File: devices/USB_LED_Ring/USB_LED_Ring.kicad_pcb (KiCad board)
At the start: 2 copper layers, 94.5 x 75 mm, 91 parts, among them J1 JST SH 3 Vert, J2 USB_B_Micro, J3 JST SH 3 Vert, J4 .100, U1 TPS923610, U2 TLV75733PDBV, U3 RP2354A, U4 TPS25947xx, Y1 ABM8-272-T3

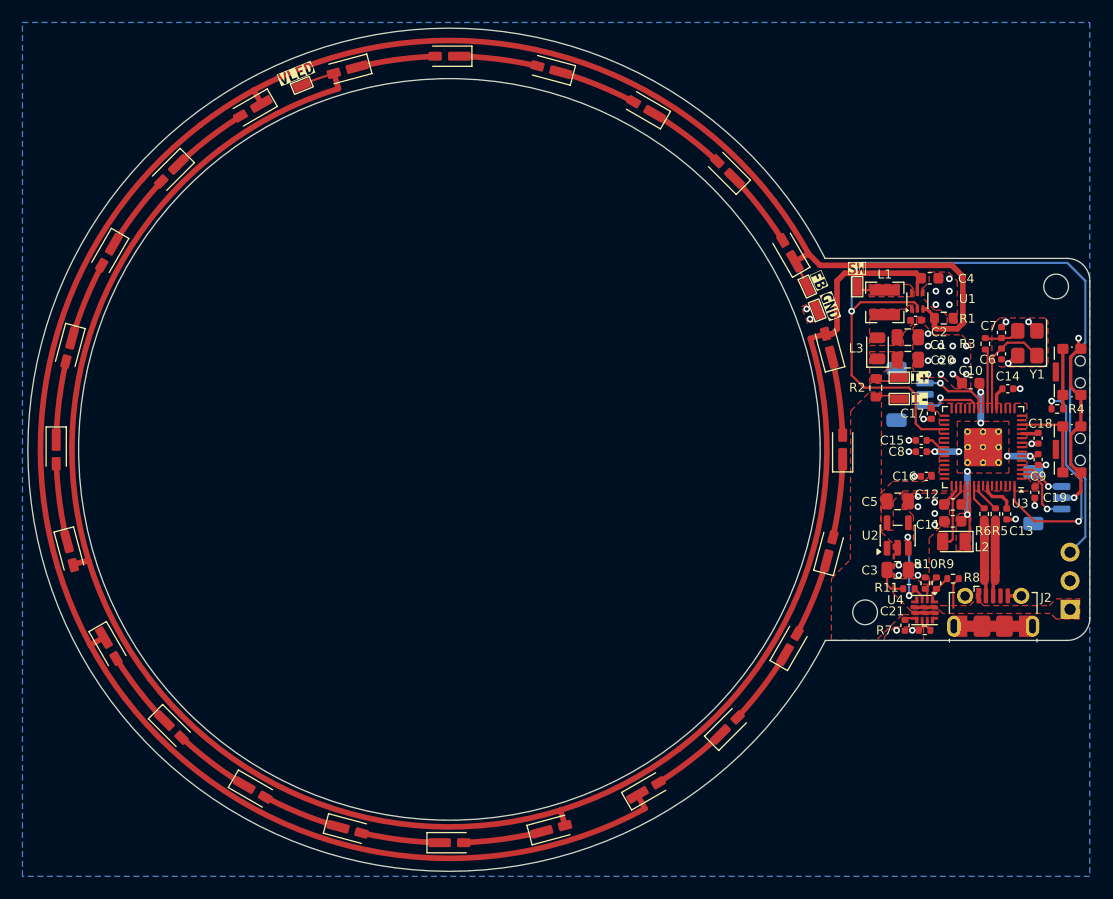
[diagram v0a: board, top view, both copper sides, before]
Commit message: Finsihes version A.0 of the BLE sensor
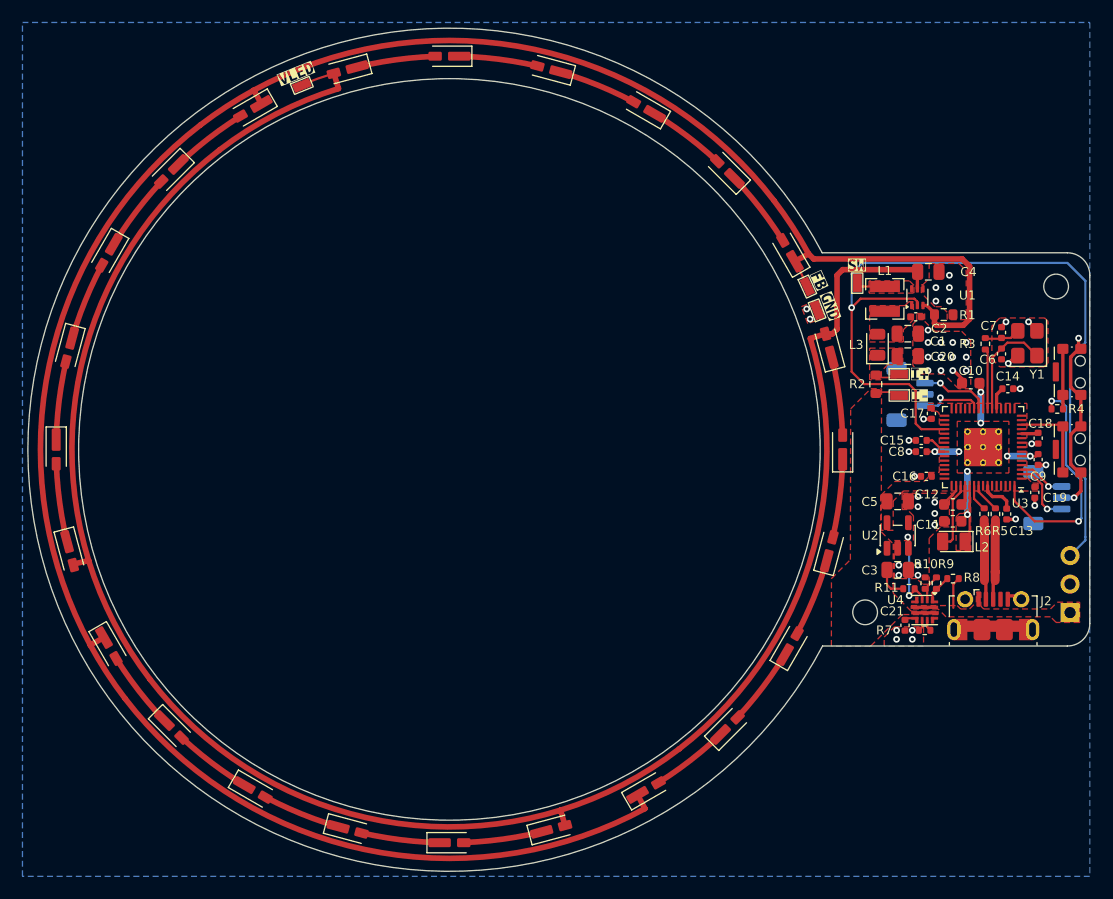
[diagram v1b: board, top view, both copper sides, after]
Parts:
- C4: value 1u -> 2u2; footprint Capacitor_SMD:C_0603_1608Metric -> Capacitor_SMD:C_0805_2012Metric
- moved C4 0.59 mm to (192.6, 84.2)
- moved C1 0.32 mm to (190.8, 89.7)
- moved C2 0.32 mm to (191.5, 88.2)
- moved C20 0.32 mm to (190.8, 91.7)
- moved L1 0.32 mm to (188.8, 86.6)
- moved L3 0.32 mm to (188.1, 90.7)
- moved R1 0.32 mm to (194.0, 88.0)
- moved R2 0.32 mm to (187.9, 94.2)
- moved TP1 0.32 mm to (186.3, 85.2)
- moved TP4 0.32 mm to (190.0, 95.2)
- moved TP5 0.32 mm to (190.0, 93.3)
- moved U1 0.32 mm to (191.7, 86.4)
- moved J2 0.30 mm to (198.4, 114.8)
- moved J4 0.30 mm to (205.2, 114.5)
- moved kibuzzard-6A117223 0.29 mm to (191.9, 95.2)
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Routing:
- net /LED_FB: track 23.7 -> 25.1 mm
- net /D+: track 6.86 -> 8.19 mm
- net /D-: track 6.84 -> 8.05 mm
- net /LED_PWM: track 75.1 -> 75.8 mm
- net GND: vias 45 -> 47
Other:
- outline, holes or cut-outs redrawn
